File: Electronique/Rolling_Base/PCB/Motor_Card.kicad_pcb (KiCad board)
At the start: 2 copper layers, 77 parts, among them K1 Maxon-200142, K2 Maxon-200142, U1 Trou-3, U10 txb0108, U11 B_Plug_5mm, U12 B_Plug_5mm, U15 txb0108, U2 Trou-3, U3 Trou-3, U4 Trou-3, U7 74HC00, U9 txb0108

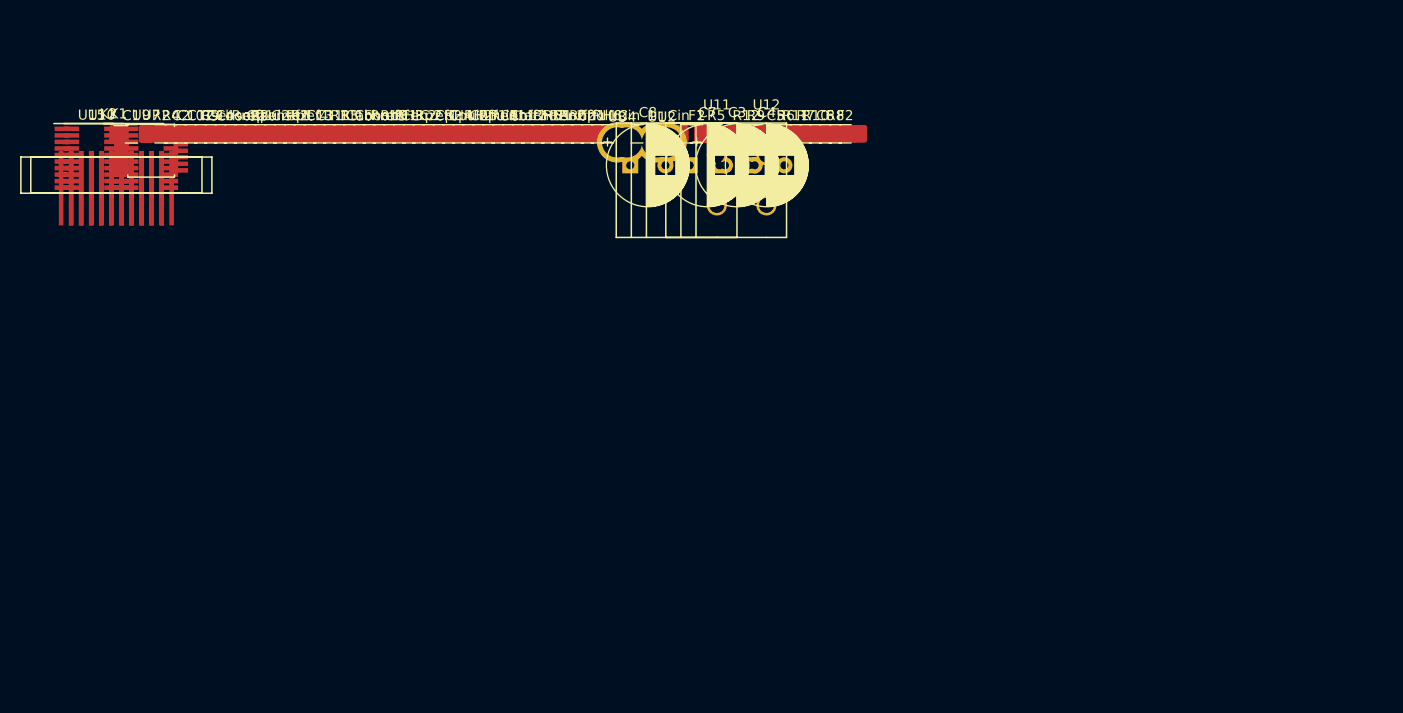
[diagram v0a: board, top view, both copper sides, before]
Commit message: Final Rolling Base Card
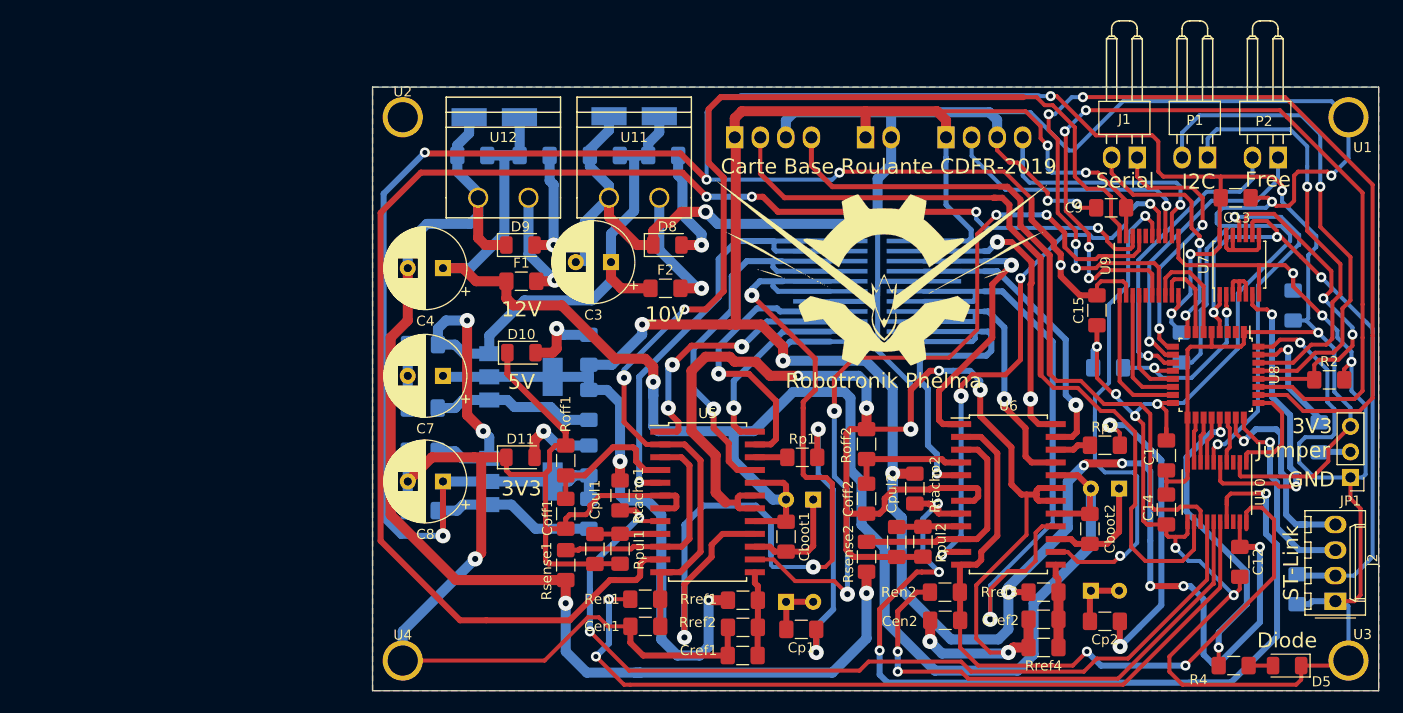
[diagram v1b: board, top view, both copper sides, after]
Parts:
- removed RH1, RH2, RH3, RH4, RH5, RH6: 10k, Resistor_SMD:R_1206_3216Metric_Pad1.42x1.75mm_HandSolder
- removed U15: txb0108, Package_SO:TSSOP-20_4.4x6.5mm_P0.65mm
- added D1: 1N4148, Diode_THT:D_DO-35_SOD27_P10.16mm_Horizontal, B.Cu at (111.1, 111.2)
- added D10: LED_5V, LED_SMD:LED_1206_3216Metric, F.Cu at (84.8, 86.4)
- added D11: LED_3.3V, LED_SMD:LED_1206_3216Metric, F.Cu at (84.7, 96.8)
- added D2: 1N4148, Diode_THT:D_DO-35_SOD27_P10.16mm_Horizontal, B.Cu at (113.8, 101.0)
- added D3: 1N4148, Diode_THT:D_DO-35_SOD27_P10.16mm_Horizontal, B.Cu at (141.4, 110.1)
- added D4: 1N4148, Diode_THT:D_DO-35_SOD27_P10.16mm_Horizontal, B.Cu at (144.2, 99.9)
- added D5: LED_ALT, LED_SMD:LED_1206_3216Metric, F.Cu at (160.9, 117.5)
- added D6: D_10A, Diode_SMD:D_SMA_Handsoldering, B.Cu at (96.0, 62.9)
- added D7: D_10A, Diode_SMD:D_SMA_Handsoldering, B.Cu at (82.1, 63.0)
- added D8: LED_VCC, LED_SMD:LED_1206_3216Metric, F.Cu at (99.3, 75.7)
- added D9: LED_ALT, LED_SMD:LED_1206_3216Metric, F.Cu at (84.7, 75.7)
- added G***: LOGO, maxon:Logo_Robotronik, F.Cu at (120.7, 77.6)
- added J1: CONN_SERIAL, Connector_Molex:Molex_KK-254_1x02_P2.54mm_Horizontal, F.Cu at (146.0, 67.0)
- added J2: swdio, Connector_Molex:Molex_KK-254_AE-6410-04A_1x04_P2.54mm_Vertical, F.Cu at (165.7, 111.1)
- added J3: FAN, Connector_Molex:Molex_KK-254_AE-6410-02A_1x02_P2.54mm_Vertical, B.Cu at (119.0, 65.0)
- added JP1: Jumper_NC_Dual, Connector_PinHeader_2.54mm:PinHeader_1x03_P2.54mm_Vertical, F.Cu at (167.2, 98.8)
- added P1: CONN_I2C, Connector_Molex:Molex_KK-254_1x02_P2.54mm_Horizontal, F.Cu at (153.0, 67.0)
- added P2: CONN_FREE, Connector_Molex:Molex_KK-254_1x02_P2.54mm_Horizontal, F.Cu at (160.0, 67.0)
- added P3: encoder_1, Connector_Molex:Molex_KK-254_AE-6410-04A_1x04_P2.54mm_Vertical, B.Cu at (127.0, 65.0)
- added P4: encoder_2, Connector_Molex:Molex_KK-254_AE-6410-04A_1x04_P2.54mm_Vertical, B.Cu at (106.0, 65.0)
- added U13: LM317_SOT223, Package_TO_SOT_SMD:SOT-223-3_TabPin2, B.Cu at (84.8, 88.8)
- added U14: LM317_SOT223, Package_TO_SOT_SMD:SOT-223-3_TabPin2, B.Cu at (84.8, 99.2)
- added U5: L6235D, Package_SO:SOIC-24W_7.5x15.4mm_P1.27mm, F.Cu at (103.3, 101.2)
- added U6: L6235D, Package_SO:SOIC-24W_7.5x15.4mm_P1.27mm, F.Cu at (133.2, 100.5)
- added U8: stm32f303k8t6, Package_QFP:LQFP-32_7x7mm_P0.8mm, F.Cu at (153.8, 88.6)
- C10, C11, C2, C5, C6, Cin_1, Cin_2, K1, K2, R1, R10, R11, R12, R3, R5, R6, R7, R8, R9: moved to B.Cu
- F1: value Fuse -> Fuse_Puiss
- F2: value Fuse -> Fuse_Num
- U11, U12: footprint B plug:B plug 5mm -> B plug:Bplug-5mm
- moved C2 119.8 mm to (161.9, 109.9), turned to 270 degrees
- moved R2 118.7 mm to (165.1, 89.1)
- moved R4 118.1 mm to (155.6, 117.5)
- moved U10 115.7 mm to (153.9, 100.2), turned to 270 degrees
- moved C12 111.7 mm to (156.2, 107.2), turned to 270 degrees
- moved U7 108.8 mm to (156.2, 77.7), turned to 90 degrees
- moved C1 107.7 mm to (148.9, 96.6), turned to 270 degrees
- moved C14 101.2 mm to (148.9, 102.0), turned to 270 degrees
- moved R3 101.0 mm to (164.1, 94.8), turned to 270 degrees
- moved U9 100.7 mm to (147.2, 77.8), turned to 90 degrees
- moved C10 100.7 mm to (150.4, 85.9), turned to 270 degrees
- moved C11 97.3 mm to (161.5, 81.7), turned to 90 degrees
- moved Cboot2 93.1 mm to (141.3, 103.9), turned to 270 degrees
- moved C13 91.3 mm to (155.8, 71.0)
- moved C9 89.8 mm to (143.4, 72.0), turned to 180 degrees
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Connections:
- C10 pad 1: +5V -> +3V3
- C9 pad 1: +3V3 -> +5V
- U10 pad 12: (no net) -> /encodeurs/Ch_A2(+5V)
- U10 pad 13: (no net) -> /encodeurs/Ch_B2(+5V)
- U10 pad 14: /encodeurs/Ch_B2(+5V) -> /motor_part/TACHO_1
- U10 pad 15: /encodeurs/Ch_A2(+5V) -> /motor_part/EN_2
- U10 pad 16: /encodeurs/Ch_B1(+5V) -> /motor_part/EN_1
- U10 pad 17: /encodeurs/Ch_A1(+5V) -> /motor_part/TACHO_2
- U10 pad 18: /motor_part/TACHO_2 -> (no net)
- U10 pad 3: /uC/Tacho_2(3V3) -> (no net)
- U10 pad 4: /encodeurs/Ch_A1 -> /uC/Tacho_2(3V3)
- U10 pad 5: /encodeurs/Ch_B1 -> Net-(U10-Pad5)
- U10 pad 6: /encodeurs/Ch_A2 -> Net-(U10-Pad6)
- U10 pad 7: /encodeurs/Ch_B2 -> /uC/Tacho_1(3V3)
- U10 pad 8: (no net) -> /encodeurs/Ch_B2
- U10 pad 9: (no net) -> /encodeurs/Ch_A2
- U7 pad 11: Net-(U7-Pad11) -> Net-(U10-Pad6)
- U7 pad 6: Net-(U7-Pad6) -> Net-(U10-Pad5)
- U9 pad 1: Net-(U7-Pad6) -> /uC/Diag_1(3V3)
- U9 pad 12: /motor_part/DIR_2 -> /encodeurs/Ch_B1(+5V)
- U9 pad 13: /motor_part/BRAKE_2 -> /encodeurs/Ch_A1(+5V)
- U9 pad 14: /motor_part/TACHO_1 -> /motor_part/DIR_2
- U9 pad 15: /motor_part/DIAG_1 -> /motor_part/BRAKE_2
- U9 pad 16: /motor_part/DIR_1 -> (no net)
- U9 pad 18: /motor_part/EN_2 -> /motor_part/DIR_1
- U9 pad 20: /motor_part/EN_1 -> /motor_part/DIAG_1
- U9 pad 3: Net-(U7-Pad11) -> /uC/Dir_1(3V3)
- U9 pad 5: /uC/Dir_1(3V3) -> (no net)
- U9 pad 6: /uC/Diag_1(3V3) -> /uC/Brake_2(3V3)
- U9 pad 7: /uC/Tacho_1(3V3) -> /uC/Dir_2(3V3)
- U9 pad 8: /uC/Brake_2(3V3) -> /encodeurs/Ch_A1
- U9 pad 9: /uC/Dir_2(3V3) -> /encodeurs/Ch_B1
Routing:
- net GND: track 0.00 -> 731.0 mm, vias 0 -> 23
- net +3V3: track 0.00 -> 318.6 mm, vias 0 -> 10
- net +5V: track 0.00 -> 303.2 mm, vias 0 -> 13
- net +12V: track 0.00 -> 166.2 mm, vias 0 -> 1
- net /motor_part/DIR_1: track 0.00 -> 149.4 mm, vias 0 -> 4
- net /motor_part/TACHO_2: track 0.00 -> 132.3 mm, vias 0 -> 4
- net GNDPWR: track 0.00 -> 120.6 mm, vias 0 -> 2
- net /motor_part/DIAG_1: track 0.00 -> 118.7 mm, vias 0 -> 2
- net /uC/Dir_2(3V3): track 0.00 -> 98.3 mm, vias 0 -> 4
- net /motor_part/Out_31: track 0.00 -> 94.1 mm, vias 0 -> 3
- net /motor_part/TACHO_1: track 0.00 -> 91.2 mm, vias 0 -> 2
- net /uC/Brake_2(3V3): track 0.00 -> 90.3 mm, vias 0 -> 4
- net /motor_part/EN_1: track 0.00 -> 82.1 mm, vias 0 -> 2
- net /encodeurs/Ch_A2(+5V): track 0.00 -> 81.9 mm
- net /motor_part/BRAKE_1: track 0.00 -> 80.0 mm, vias 0 -> 4
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- added copper zone on B.Cu, net GND
- added copper zone on F.Cu, net GND
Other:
- board outline added: 100 x 60 mm
- net class Alimentation added: clearance 0.2, trace_width 1, via_dia 1.5, via_drill 0.6
- net class Default: trace_width 0.25 -> 0.4; via_dia 0.8 -> 1; via_drill 0.4 -> 0.5
- rule trace_min: 0.2 -> 0.4
- rule via_min_size: 0.4 -> 0.5
- board text added: "10V"
- board text added: "12V"
- board text added: "3V3"
- board text added: "5V"
- board text added: "Carte Base Roulante CDFR-2019"
- board text added: "Diode"
- board text added: "Encodeur-1"
- board text added: "Encodeur-2"
- board text added: "Free"
- board text added: "GND"
- board text added: "I2C"
- board text added: "Jumper"
- board text added: "Moteur-1"
- board text added: "Moteur-2"
- board text added: "Robotronik Phelma"
- board text added: "ST-Link"
- board text added: "Serial"
